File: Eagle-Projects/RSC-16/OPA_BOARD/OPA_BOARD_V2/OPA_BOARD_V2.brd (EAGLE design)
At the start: 63.5 x 53 mm, 19 parts

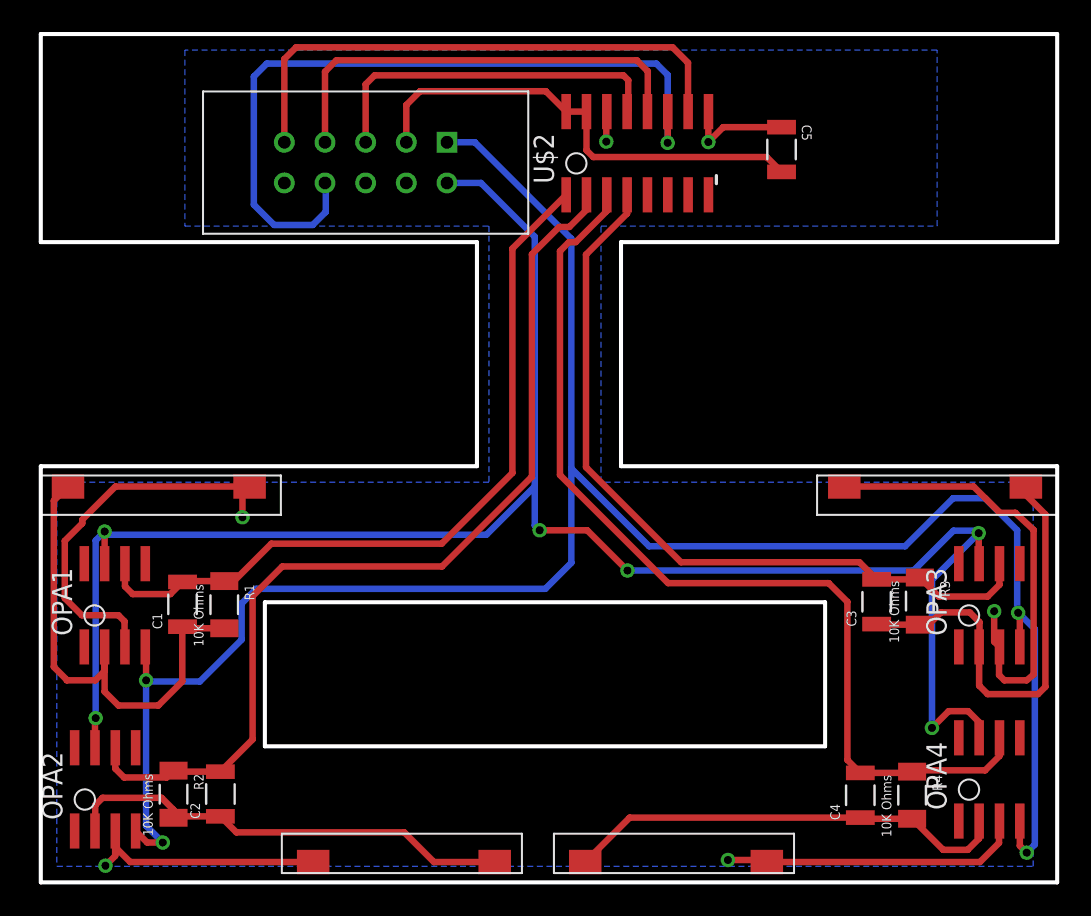
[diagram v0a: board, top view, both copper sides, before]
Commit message: Commit of all RockSat-C 2016 payload designs.
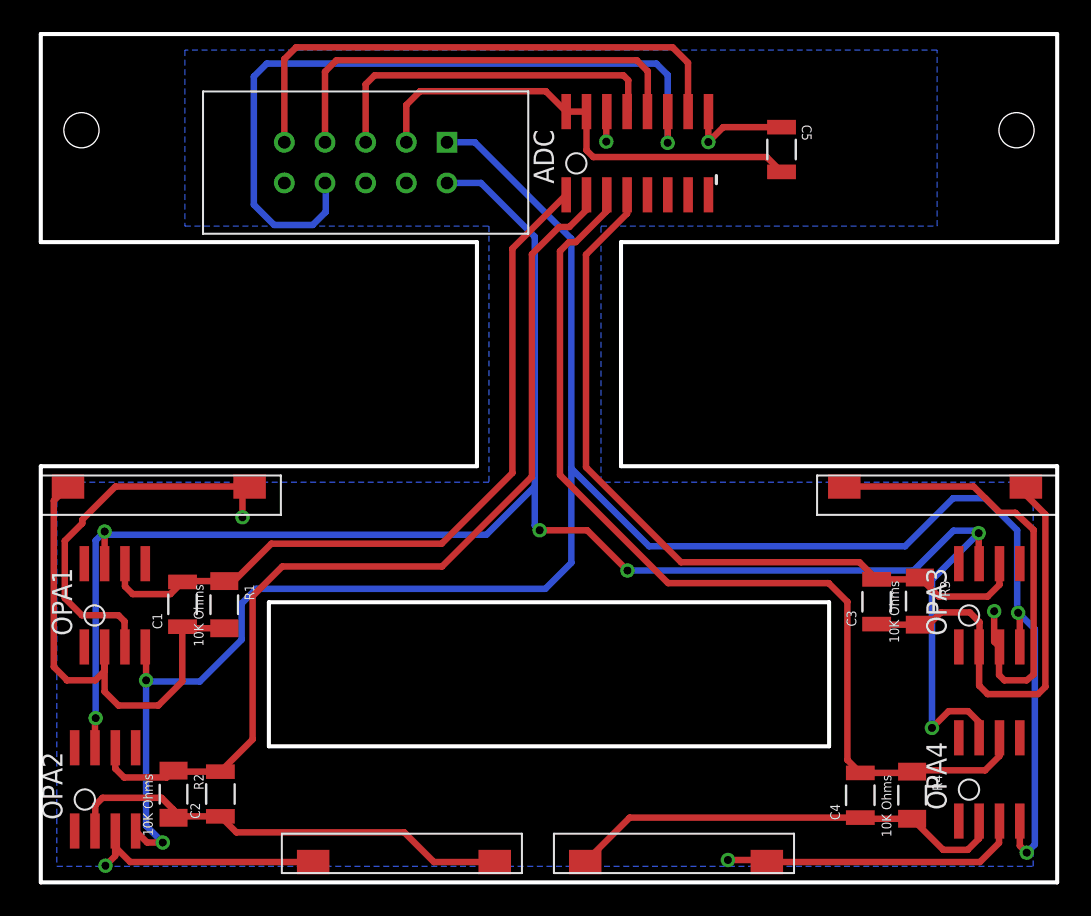
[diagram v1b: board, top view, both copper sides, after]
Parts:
- ADC: value MCP3008-SOIC16 -> (none)
- renumbered U$2 to ADC
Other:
- outline, holes or cut-outs redrawn
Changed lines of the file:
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@@
 <setting verticaltext="up"/>
 </settings>
-<grid distance="0.01" unitdist="inch" unit="inch" style="lines" multiple="1" display="yes" altdistance="1" altunitdist="mil" altunit="mil"/>
+<grid distance="0.1" unitdist="inch" unit="inch" style="lines" multiple="1" display="yes" altdistance="0.05" altunitdist="inch" altunit="inch"/>
 <layers>
 <layer number="1" name="Top" color="4" fill="1" visible="yes" active="yes"/>
@@
 <wire x1="27.25" y1="26" x2="0" y2="26" width="0.254" layer="20"/>
 <wire x1="0" y1="26" x2="0" y2="0" width="0.254" layer="20"/>
-<wire x1="14" y1="8.5" x2="49" y2="8.5" width="0.254" layer="20"/>
-<wire x1="49" y1="8.5" x2="49" y2="17.5" width="0.254" layer="20"/>
-<wire x1="49" y1="17.5" x2="14" y2="17.5" width="0.254" layer="20"/>
-<wire x1="14" y1="17.5" x2="14" y2="8.5" width="0.254" layer="20"/>
+<wire x1="14.25" y1="8.5" x2="49.25" y2="8.5" width="0.254" layer="20"/>
+<wire x1="49.25" y1="8.5" x2="49.25" y2="17.5" width="0.254" layer="20"/>
+<wire x1="49.25" y1="17.5" x2="14.25" y2="17.5" width="0.254" layer="20"/>
+<wire x1="14.25" y1="17.5" x2="14.25" y2="8.5" width="0.254" layer="20"/>
+<hole x="2.54" y="46.99" drill="2.2"/>
+<hole x="60.96" y="46.99" drill="2.2"/>
 </plain>
 <attributes>
@@
 <attribute name="SUPPLIER" value="Kemet" x="46.2792" y="45.7862" size="1.778" layer="27" rot="R270" display="off"/>
 </element>
-<element name="U$2" library="RSC-16" package="SOIC16N" value="MCP3008-SOIC16" x="37.268" y="45.5554"/>
+<element name="ADC" library="RSC-16" package="SOIC16N" value="" x="37.268" y="45.5554"/>
 </elements>
 <signals>
@@
 <wire x1="59.1566" y1="17.8562" x2="56.1076" y2="17.8562" width="0.4064" layer="1"/>
 <wire x1="56.1076" y1="17.8562" x2="54.9182" y2="19.0456" width="0.4064" layer="1"/>
-<contactref element="U$2" pad="4"/>
+<contactref element="ADC" pad="4"/>
 <wire x1="36.633" y1="42.9554" x2="36.633" y2="41.7892" width="0.4064" layer="1"/>
 <wire x1="36.633" y1="41.7892" x2="34.0614" y2="39.2176" width="0.4064" layer="1"/>
@@
 <wire x1="5.207" y1="6.5532" x2="7.8656" y2="6.5532" width="0.4064" layer="1"/>
 <wire x1="7.8656" y1="6.5532" x2="8.2938" y2="6.9814" width="0.4064" layer="1"/>
-<contactref element="U$2" pad="2"/>
+<contactref element="ADC" pad="2"/>
 <wire x1="34.093" y1="42.9554" x2="34.093" y2="42.0178" width="0.4064" layer="1"/>
 <wire x1="34.093" y1="42.0178" x2="33.02" y2="40.9448" width="0.4064" layer="1"/>
@@
 <wire x1="59" y1="7" x2="54.519" y2="7" width="0.4064" layer="1"/>
 <wire x1="54.519" y1="7" x2="54.437" y2="6.918" width="0.4064" layer="1"/>
-<contactref element="U$2" pad="3"/>
+<contactref element="ADC" pad="3"/>
 <wire x1="32.4358" y1="25.4508" x2="39.1922" y2="18.6944" width="0.4064" layer="1"/>
 <wire x1="39.1922" y1="18.6944" x2="49.2252" y2="18.6944" width="0.4064" layer="1"/>
@@
 <wire x1="11.4622" y1="18.8218" x2="8.9084" y2="18.8218" width="0.4064" layer="1"/>
 <wire x1="8.9084" y1="18.8218" x2="8.855" y2="18.7684" width="0.4064" layer="1"/>
-<contactref element="U$2" pad="1"/>
+<contactref element="ADC" pad="1"/>
 <wire x1="11.4622" y1="18.8218" x2="12.0654" y2="18.8218" width="0.4064" layer="1"/>
 <wire x1="12.0654" y1="18.8218" x2="14.4018" y2="21.1582" width="0.4064" layer="1"/>
@@
 <contactref element="U$1" pad="6-GND"/>
 <contactref element="C5" pad="1"/>
-<contactref element="U$2" pad="14"/>
-<contactref element="U$2" pad="9"/>
+<contactref element="ADC" pad="14"/>
+<contactref element="ADC" pad="9"/>
 <via x="35.3314" y="46.2788" extent="1-16" drill="0.5" shape="square"/>
 <via x="41.7068" y="46.2534" extent="1-16" drill="0.5" shape="square"/>
@@
 <signal name="MOSI">
 <contactref element="U$1" pad="7-MOSI"/>
-<contactref element="U$2" pad="11"/>
+<contactref element="ADC" pad="11"/>
 <via x="39.1668" y="46.2026" extent="1-16" drill="0.5" shape="square"/>
 <wire x1="39.1668" y1="46.2026" x2="39.1668" y2="50.4444" width="0.4064" layer="16"/>
@@
 <contactref element="U$1" pad="2-5V"/>
 <contactref element="C5" pad="2"/>
-<contactref element="U$2" pad="16"/>
-<contactref element="U$2" pad="15"/>
+<contactref element="ADC" pad="16"/>
+<contactref element="ADC" pad="15"/>
 <wire x1="22.8354" y1="46.238" x2="22.8354" y2="48.5656" width="0.4064" layer="1"/>
 <wire x1="22.8354" y1="48.5656" x2="23.6982" y2="49.4284" width="0.4064" layer="1"/>
@@
 <signal name="SCLK">
 <contactref element="U$1" pad="3-SCLK"/>
-<contactref element="U$2" pad="13"/>
+<contactref element="ADC" pad="13"/>
 <wire x1="20.2954" y1="46.238" x2="20.2954" y2="49.861" width="0.4064" layer="1"/>
 <wire x1="20.2954" y1="49.861" x2="20.8534" y2="50.419" width="0.4064" layer="1"/>
@@
 <signal name="MISO">
 <contactref element="U$1" pad="4-MISO"/>
-<contactref element="U$2" pad="12"/>
+<contactref element="ADC" pad="12"/>
 <wire x1="17.7554" y1="46.238" x2="17.7554" y2="50.6484" width="0.4064" layer="1"/>
 <wire x1="17.7554" y1="50.6484" x2="18.4658" y2="51.3588" width="0.4064" layer="1"/>
@@
 <signal name="CS">
 <contactref element="U$1" pad="5-CS"/>
-<contactref element="U$2" pad="10"/>
+<contactref element="ADC" pad="10"/>
 <wire x1="15.2154" y1="46.238" x2="15.2154" y2="51.4358" width="0.4064" layer="1"/>
 <wire x1="15.2154" y1="51.4358" x2="15.9512" y2="52.1716" width="0.4064" layer="1"/>
